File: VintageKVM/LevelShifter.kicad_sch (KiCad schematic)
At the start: 5 parts, among them Q1 BSS138

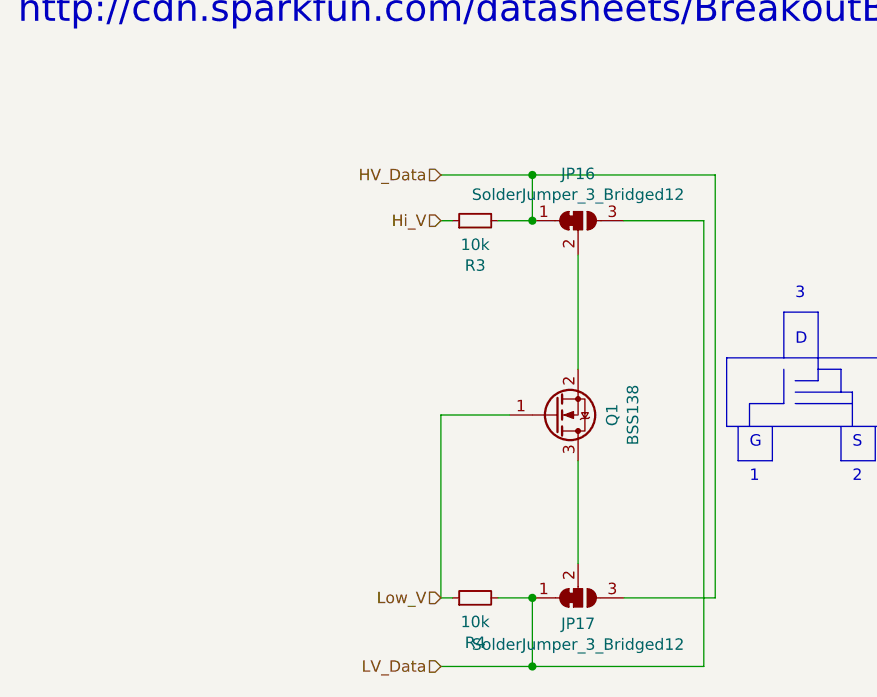
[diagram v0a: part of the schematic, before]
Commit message: routing complete
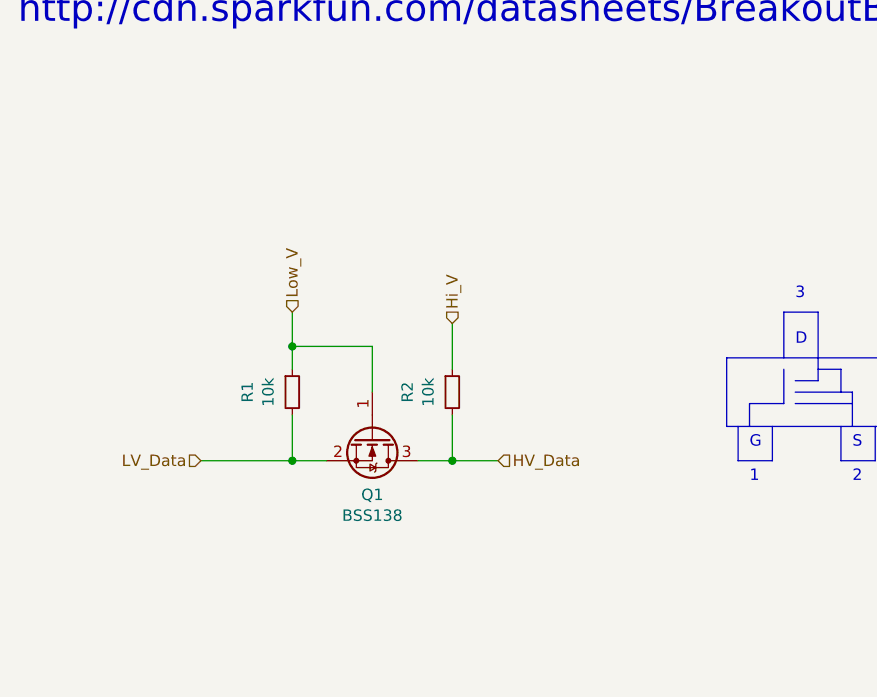
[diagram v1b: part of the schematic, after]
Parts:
- removed JP16, JP17: SolderJumper_3_Bridged12, Jumper:SolderJumper-3_P1.3mm_Bridged12_RoundedPad1.0x1.5mm, symbol Jumper:SolderJumper_3_Bridged12
- Q1: LCSC C52895 -> C78284
- renumbered R4 to R1, R3 to R2
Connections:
- net HV_Data: now also Q1.3 (D)
- net LV_Data: now also Q1.2 (S)
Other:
- moved on the sheet: Q1, R1, R2
